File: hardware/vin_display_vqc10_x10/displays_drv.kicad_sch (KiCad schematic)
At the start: 38 parts, among them Q2 DMP2022LSS, Q3 DMP2022LSS, Q4 DMP2022LSS, Q5 DMP2022LSS, Q6 DMP2022LSS, Q8 DMP2022LSS, Q9 DMP2022LSS, U14 74HCT154, U15 74HCT154, U16 74HCT154

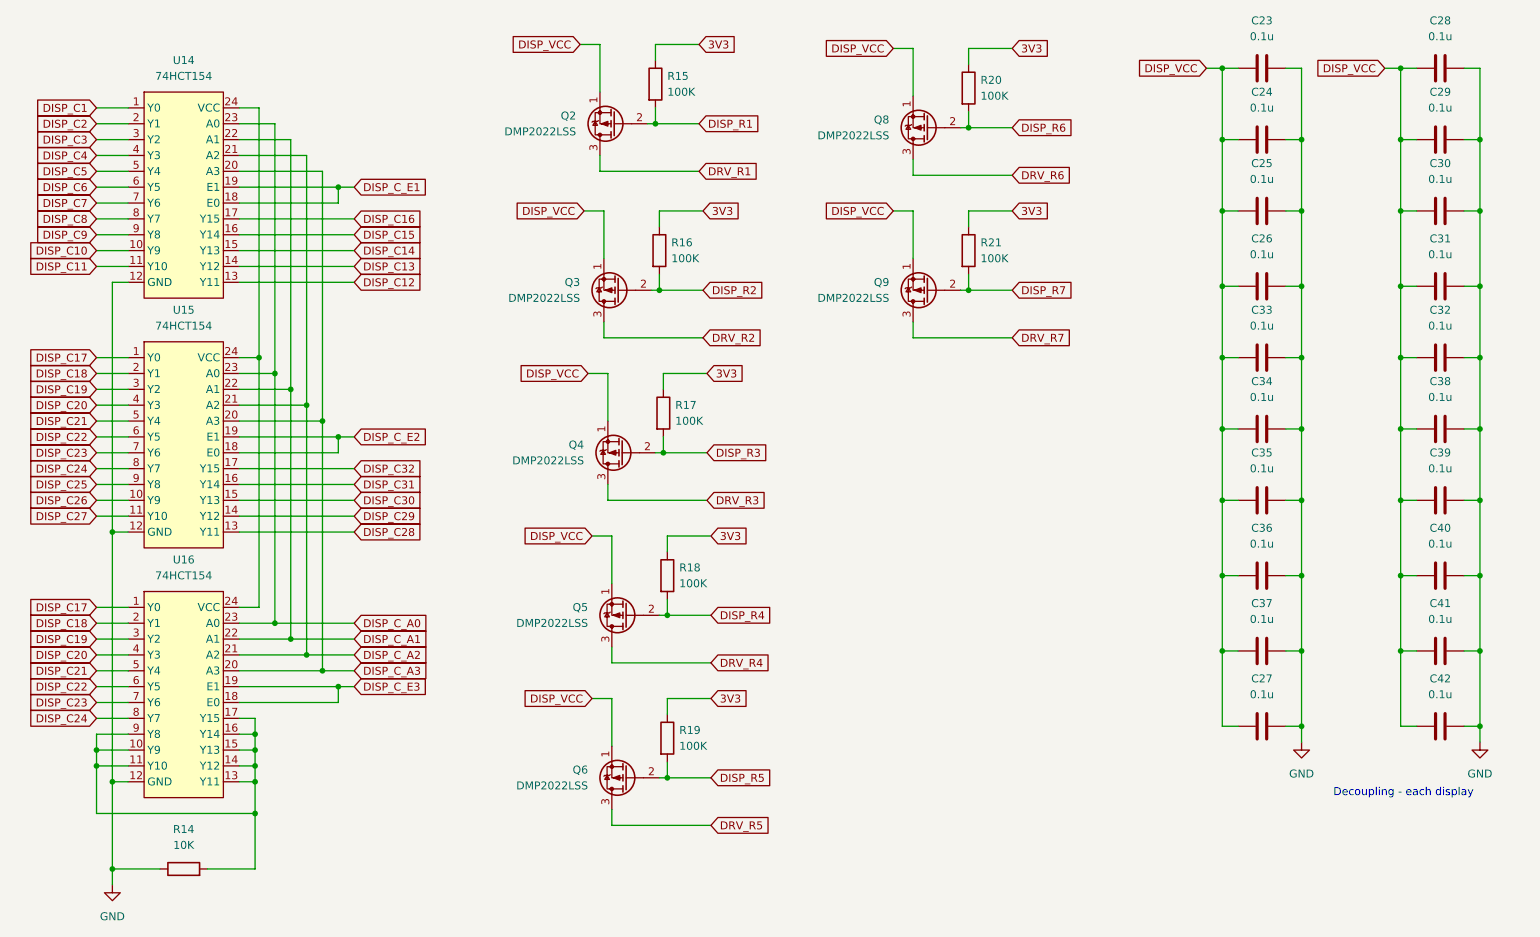
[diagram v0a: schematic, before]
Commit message: routing vqc10_x10
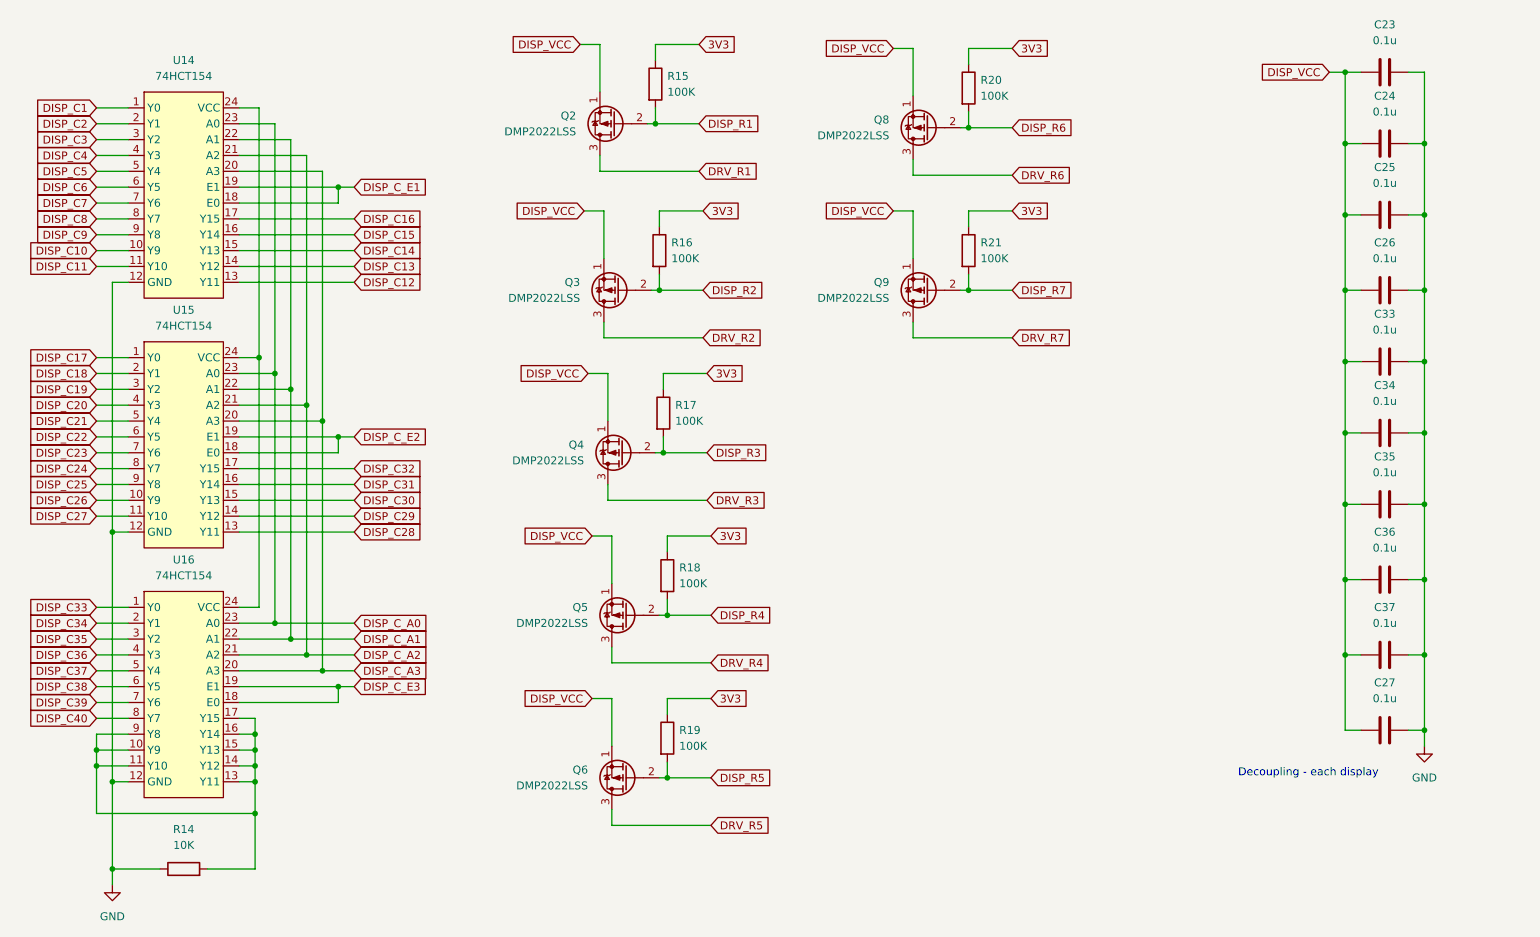
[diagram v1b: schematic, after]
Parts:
- removed C28, C29, C30, C31, C32, C38, C39, C40, C41, C42: 0.1u, Capacitor_SMD:C_0603_1608Metric, symbol Device:C
- R14: footprint (none) -> Capacitor_SMD:C_0603_1608Metric
- U14, U15, U16: footprint (none) -> Package_SO:TSSOP-24_4.4x7.8mm_P0.65mm
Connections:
- net DISP_C17: no longer U16.1 (Y0)
- net DISP_C18: no longer U16.2 (Y1)
- net DISP_C19: no longer U16.3 (Y2)
- net DISP_C20: no longer U16.4 (Y3)
- net DISP_C21: no longer U16.5 (Y4)
- net DISP_C22: no longer U16.6 (Y5)
- net DISP_C23: no longer U16.7 (Y6)
- net DISP_C24: no longer U16.8 (Y7)
- new net DISP_C33: U16.1 (Y0)
- new net DISP_C34: U16.2 (Y1)
- new net DISP_C35: U16.3 (Y2)
- new net DISP_C36: U16.4 (Y3)
- new net DISP_C37: U16.5 (Y4)
- new net DISP_C38: U16.6 (Y5)
- new net DISP_C39: U16.7 (Y6)
- new net DISP_C40: U16.8 (Y7)
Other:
- moved on the sheet: C23, C24, C25, C26, C27, C33, C34, C35, C36, C37

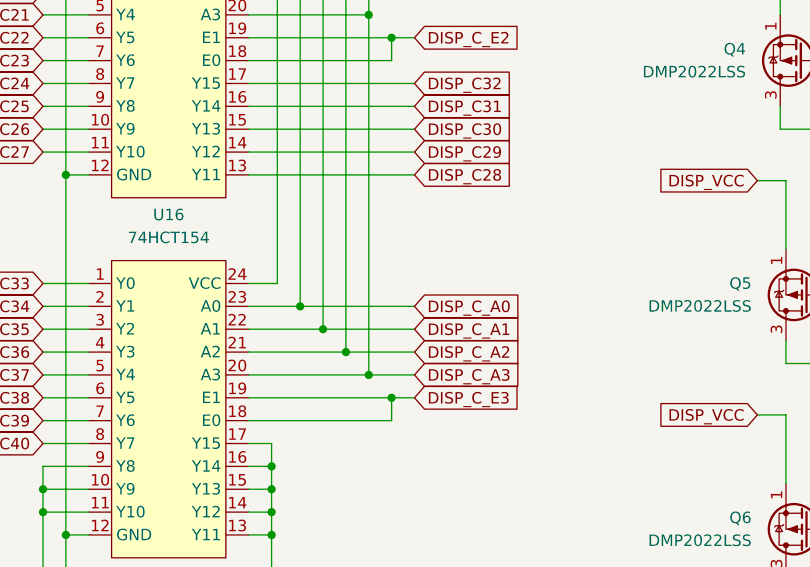
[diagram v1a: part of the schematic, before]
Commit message: route vqc10_x10 board
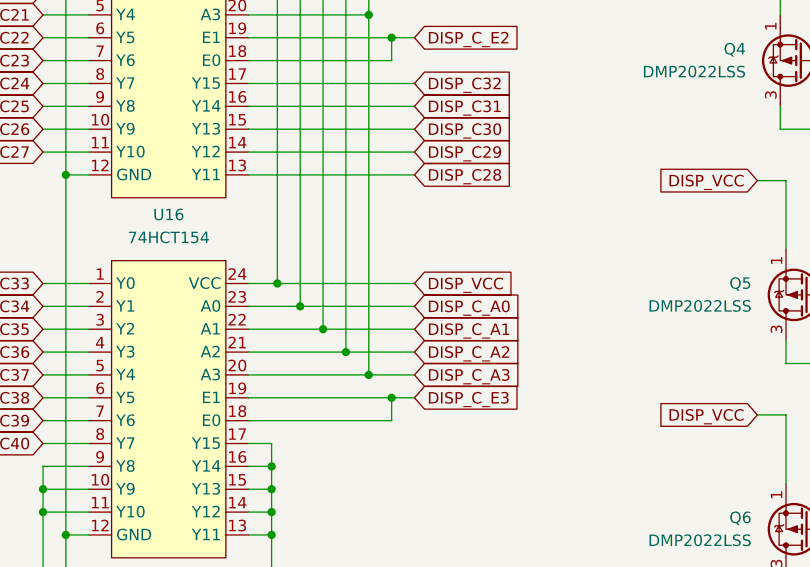
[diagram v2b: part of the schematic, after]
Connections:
- net DISP_VCC: now also U14.24 (VCC), U15.24 (VCC), U16.24 (VCC)
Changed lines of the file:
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@@
   (junction (at 250.19 97.79) (diameter 0) (color 0 0 0 0)
   )
+  (junction (at 63.5 114.3) (diameter 0) (color 0 0 0 0)
+  )
   (junction (at 73.66 84.455) (diameter 0) (color 0 0 0 0)
   )
@@
   )
   (wire (pts (xy 127.635 50.8) (xy 127.635 53.34))
+    (stroke (width 0) (type default))
+  )
+  (wire (pts (xy 63.5 114.3) (xy 78.74 114.3))
     (stroke (width 0) (type default))
   )
@@
       (effects (font (size 1.27 1.27)) (justify left) hide)
     )
+  )
+  (global_label "DISP_VCC" (shape input) (at 78.74 114.3 0) (fields_autoplaced)
+    (effects (font (size 1.27 1.27)) (justify left))
+    (property "Intersheetrefs" "${INTERSHEET_REFS}" (at 90.6757 114.3 0)
+      (effects (font (size 1.27 1.27)) (justify left) hide)
+    )
